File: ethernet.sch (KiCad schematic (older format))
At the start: 24 parts, among them J3 L834-1G1T-91, U9 KSZ8081RNA, Y3 25M

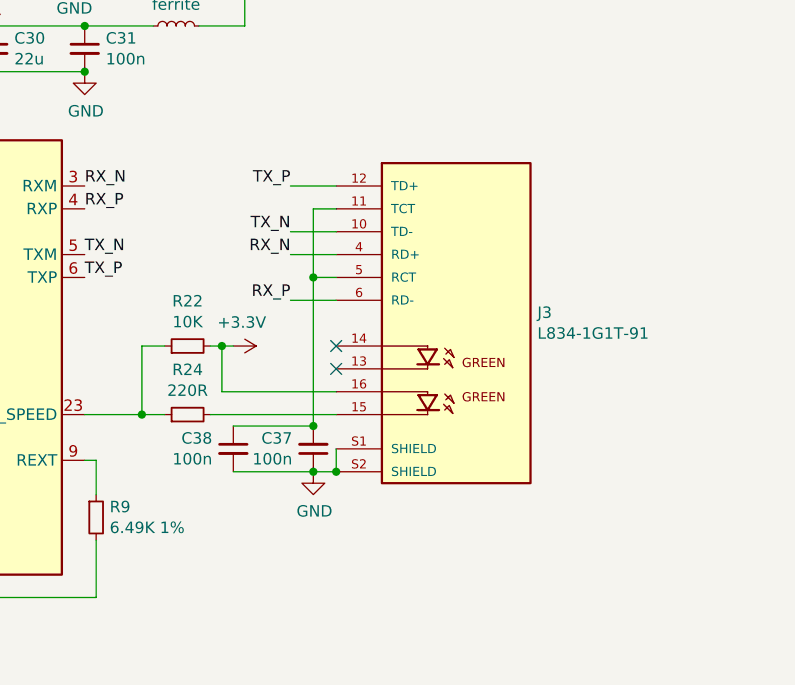
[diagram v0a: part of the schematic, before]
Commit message: Save point
Signed-off-by: Martin Ribelotta <martinribelotta@gmail.com>
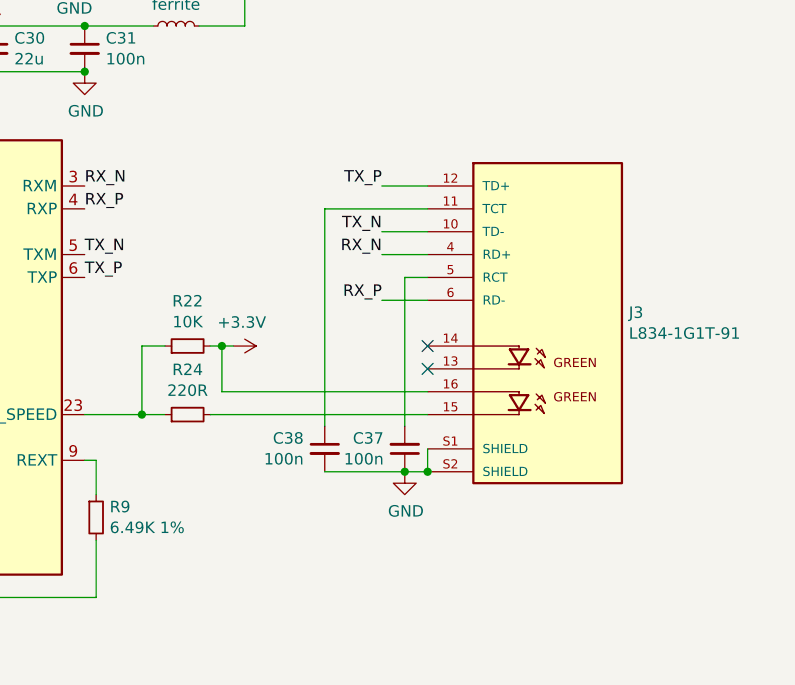
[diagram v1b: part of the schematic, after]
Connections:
- net at C37.2, J3.5 (RCT): no longer C38.1, J3.11 (TCT)
- new net: C38.1, J3.11 (TCT)
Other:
- moved on the sheet: C37, C38, J3
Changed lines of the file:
@@
 Comment4 ""
 $EndDescr
-Wire Wire Line
-	7500 3600 7400 3600
 $Comp
 L Device:C_Small C?
 U 1 1 6019A4E1
-P 7400 4650
+P 7800 4650
 AR Path="/6019A4E1" Ref="C?"  Part="1"
 AR Path="/60185BCA/6019A4E1" Ref="C37"  Part="1"
-F 0 "C37" H 7308 4604 50  0000 R CNN
-F 1 "100n" H 7308 4695 50  0000 R CNN
-F 2 "Capacitor_SMD:C_0603_1608Metric" H 7400 4650 50  0001 C CNN
-F 3 "~" H 7400 4650 50  0001 C CNN
-F 4 "Capacitor 0.022u 0603" H 7400 4650 50  0001 C CNN "DESCRIPTION"
-F 5 "AVX" H 7400 4650 50  0001 C CNN "MANUFACTURER"
-F 6 "06035C223KAT2A" H 7400 4650 50  0001 C CNN "MANUFACTURER_PART_NUMBER"
-	1    7400 4650
+F 0 "C37" H 7708 4604 50  0000 R CNN
+F 1 "100n" H 7708 4695 50  0000 R CNN
+F 2 "Capacitor_SMD:C_0603_1608Metric" H 7800 4650 50  0001 C CNN
+F 3 "~" H 7800 4650 50  0001 C CNN
+F 4 "Capacitor 0.022u 0603" H 7800 4650 50  0001 C CNN "DESCRIPTION"
+F 5 "AVX" H 7800 4650 50  0001 C CNN "MANUFACTURER"
+F 6 "06035C223KAT2A" H 7800 4650 50  0001 C CNN "MANUFACTURER_PART_NUMBER"
+	1    7800 4650
 	1    0    0    1
 $EndComp
@@
 L power:GND #PWR050
 U 1 1 6019B07E
-P 7400 4750
-F 0 "#PWR050" H 7400 4500 50  0001 C CNN
-F 1 "GND" H 7405 4577 50  0000 C CNN
-F 2 "" H 7400 4750 50  0001 C CNN
-F 3 "" H 7400 4750 50  0001 C CNN
-	1    7400 4750
+P 7800 4750
+F 0 "#PWR050" H 7800 4500 50  0001 C CNN
+F 1 "GND" H 7805 4577 50  0000 C CNN
+F 2 "" H 7800 4750 50  0001 C CNN
+F 3 "" H 7800 4750 50  0001 C CNN
+	1    7800 4750
 	1    0    0    -1
 $EndComp
@@
 	1    0    0    -1
 $EndComp
-Connection ~ 7400 4750
+Connection ~ 7800 4750
 Wire Wire Line
 	4500 5450 4300 5450
@@
 Connection ~ 6400 3000
 Wire Wire Line
-	7050 4550 7400 4550
-Connection ~ 7400 4550
-Wire Wire Line
-	7400 4750 7050 4750
-Wire Wire Line
-	7400 3600 7400 3900
-Wire Wire Line
-	7500 3900 7400 3900
-Connection ~ 7400 3900
-Wire Wire Line
-	7400 3900 7400 4550
+	7800 4750 7450 4750
+Wire Wire Line
+	7900 3900 7800 3900
+Wire Wire Line
+	7800 3900 7800 4550
 $Comp
 L Device:C_Small C?
 U 1 1 6045B459
-P 7050 4650
+P 7450 4650
 AR Path="/6045B459" Ref="C?"  Part="1"
 AR Path="/60185BCA/6045B459" Ref="C38"  Part="1"
-F 0 "C38" H 7142 4696 50  0000 L CNN
-F 1 "100n" H 7142 4605 50  0000 L CNN
-F 2 "Capacitor_SMD:C_0603_1608Metric" H 7050 4650 50  0001 C CNN
-F 3 "~" H 7050 4650 50  0001 C CNN
-F 4 "Capacitor 0.022u 0603" H 7050 4650 50  0001 C CNN "DESCRIPTION"
-F 5 "AVX" H 7050 4650 50  0001 C CNN "MANUFACTURER"
-F 6 "06035C223KAT2A" H 7050 4650 50  0001 C CNN "MANUFACTURER_PART_NUMBER"
-	1    7050 4650
+F 0 "C38" H 7542 4696 50  0000 L CNN
+F 1 "100n" H 7542 4605 50  0000 L CNN
+F 2 "Capacitor_SMD:C_0603_1608Metric" H 7450 4650 50  0001 C CNN
+F 3 "~" H 7450 4650 50  0001 C CNN
+F 4 "Capacitor 0.022u 0603" H 7450 4650 50  0001 C CNN "DESCRIPTION"
+F 5 "AVX" H 7450 4650 50  0001 C CNN "MANUFACTURER"
+F 6 "06035C223KAT2A" H 7450 4650 50  0001 C CNN "MANUFACTURER_PART_NUMBER"
+	1    7450 4650
 	-1   0    0    -1
 $EndComp
@@
 L L834-1G1T-91:L834-1G1T-91 J3
 U 1 1 6064910E
-P 8000 4100
-F 0 "J3" H 8380 4146 50  0000 L CNN
-F 1 "L834-1G1T-91" H 8380 4055 50  0000 L CNN
-F 2 "footprints:BEL_L834-1G1T-91" H 8000 4100 50  0001 L BNN
-F 3 "" H 8000 4100 50  0001 L BNN
-F 4 "Bel Fuse" H 8000 4100 50  0001 L BNN "MANUFACTURER"
-F 5 "Manufacturer Recommendations" H 8000 4100 50  0001 L BNN "STANDARD"
-F 6 "C" H 8000 4100 50  0001 L BNN "PARTREV"
-F 7 "11.46 mm" H 8000 4100 50  0001 L BNN "MAXIMUM_PACKAGE_HEIGHT"
-F 8 "L834-1G1T-91" H 8000 4100 50  0001 C CNN "MANUFACTURER_PART_NUMBER"
-	1    8000 4100
-	1    0    0    -1
-$EndComp
-Wire Wire Line
-	7500 4750 7400 4750
-Wire Wire Line
-	7500 4650 7500 4750
-Connection ~ 7500 4750
+P 8400 4100
+F 0 "J3" H 8780 4146 50  0000 L CNN
+F 1 "L834-1G1T-91" H 8780 4055 50  0000 L CNN
+F 2 "footprints:BEL_L834-1G1T-91" H 8400 4100 50  0001 L BNN
+F 3 "" H 8400 4100 50  0001 L BNN
+F 4 "Bel Fuse" H 8400 4100 50  0001 L BNN "MANUFACTURER"
+F 5 "Manufacturer Recommendations" H 8400 4100 50  0001 L BNN "STANDARD"
+F 6 "C" H 8400 4100 50  0001 L BNN "PARTREV"
+F 7 "11.46 mm" H 8400 4100 50  0001 L BNN "MAXIMUM_PACKAGE_HEIGHT"
+F 8 "L834-1G1T-91" H 8400 4100 50  0001 C CNN "MANUFACTURER_PART_NUMBER"
+	1    8400 4100
+	1    0    0    -1
+$EndComp
+Wire Wire Line
+	7900 4750 7800 4750
+Wire Wire Line
+	7900 4650 7900 4750
+Connection ~ 7900 4750
 $Comp
 L Device:R_Small R?
@@
 Wire Wire Line
 	5600 2050 5600 3200
-Text Label 7300 3500 2    50   ~ 0
+Text Label 7700 3500 2    50   ~ 0
 TX_P
-Text Label 7300 3700 2    50   ~ 0
+Text Label 7700 3700 2    50   ~ 0
 TX_N
-Text Label 7300 4000 2    50   ~ 0
+Text Label 7700 4000 2    50   ~ 0
 RX_P
-Text Label 7300 3800 2    50   ~ 0
+Text Label 7700 3800 2    50   ~ 0
 RX_N
 Wire Wire Line
-	7300 4000 7500 4000
-Wire Wire Line
-	7500 3800 7300 3800
-Wire Wire Line
-	7300 3500 7500 3500
-Wire Wire Line
-	7500 3700 7300 3700
-NoConn ~ 7500 4300
-NoConn ~ 7500 4200
+	7700 4000 7900 4000
+Wire Wire Line
+	7900 3800 7700 3800
+Wire Wire Line
+	7700 3500 7900 3500
+Wire Wire Line
+	7900 3700 7700 3700
+NoConn ~ 7900 4300
+NoConn ~ 7900 4200
 Wire Wire Line
 	6400 4700 6450 4700
@@
 	6450 5300 6450 5050
 Connection ~ 5700 5300
-Wire Wire Line
-	6950 4500 7500 4500
 Wire Wire Line
 	6400 4500 6650 4500
@@
 Wire Wire Line
 	7000 4200 7000 4400
-Wire Wire Line
-	7000 4400 7500 4400
 Connection ~ 7000 4200
 Wire Wire Line
@@
 	4300 5000 4300 5100
 Connection ~ 4300 5100
+Wire Wire Line
+	6950 4500 7900 4500
+Wire Wire Line
+	7000 4400 7900 4400
+Wire Wire Line
+	7450 4550 7450 3600
+Wire Wire Line
+	7450 3600 7900 3600
 $EndSCHEMATC
